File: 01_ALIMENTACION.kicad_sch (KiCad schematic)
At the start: 7 parts, among them J2 DC-005-5A-2.0, Q1 IRFR5305TRPBF, Q2 IRFR5305TRPBF

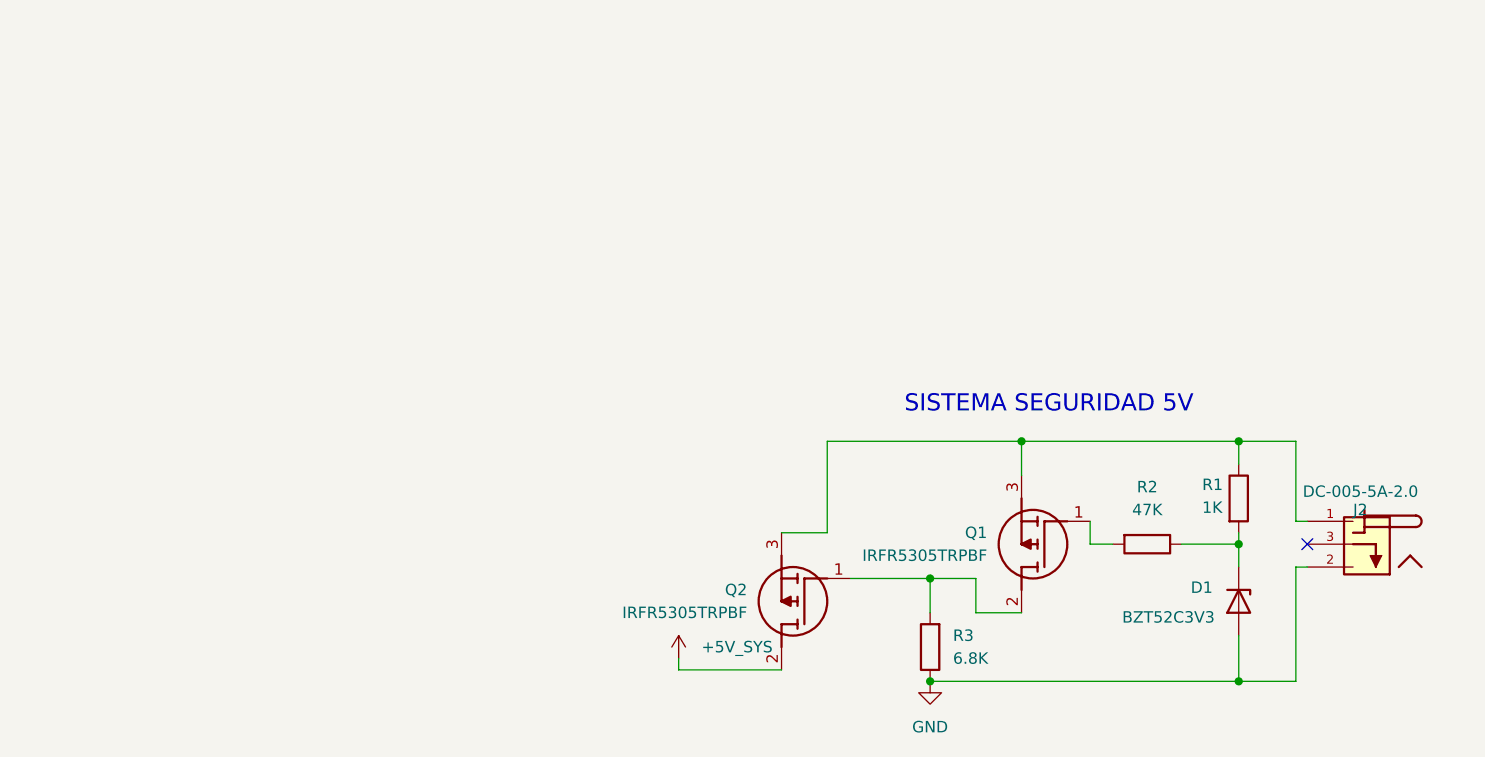
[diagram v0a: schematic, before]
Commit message: Added IMU
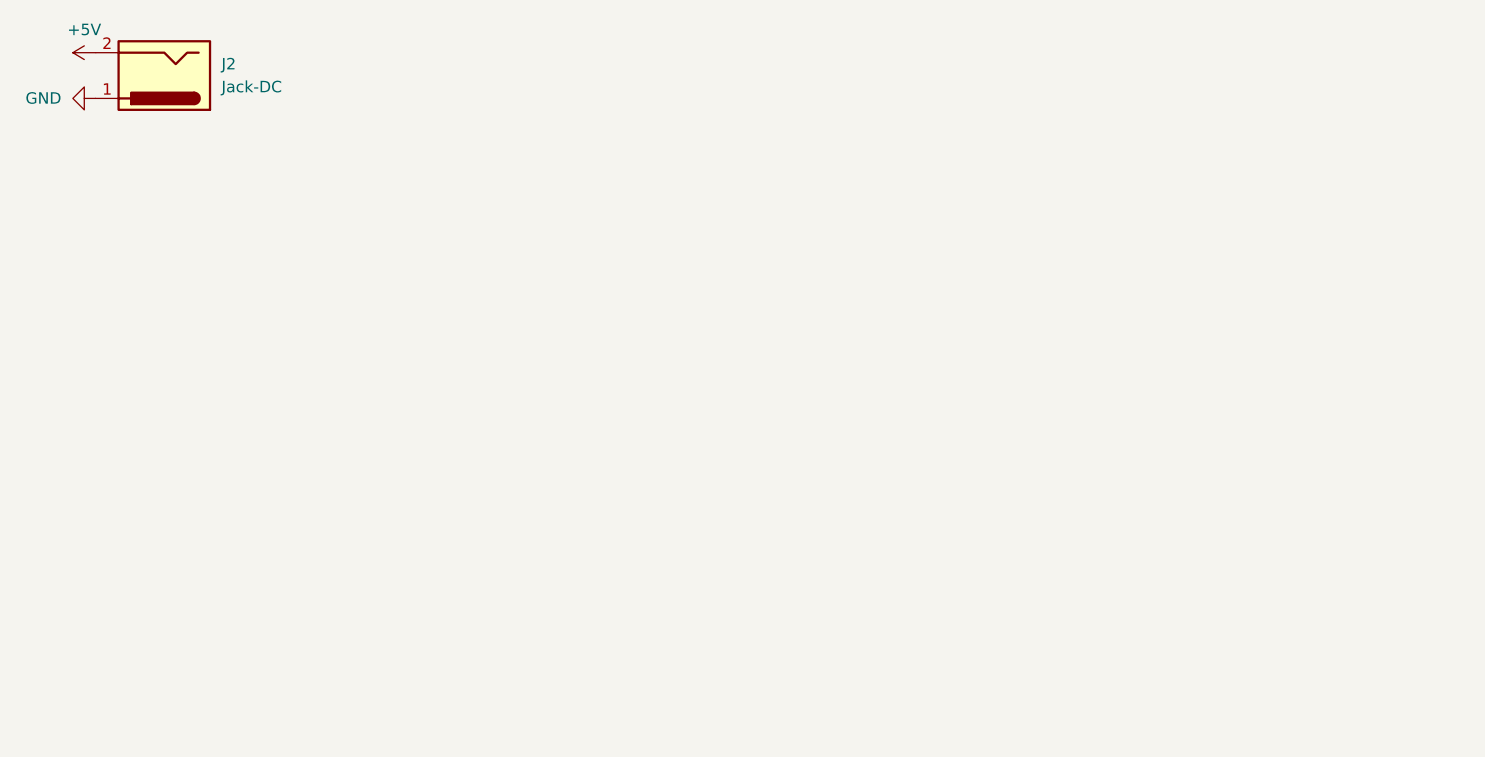
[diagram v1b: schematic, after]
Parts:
- removed D1: BZT52C3V3, Footprints:SOD3715X135N, symbol Device:D_Zener
- removed J2: DC-005-5A-2.0, Footprints:XKB_DC-005-5A-2.0, symbol Simbolos:DC-005-5A-2.0
- removed Q1, Q2: IRFR5305TRPBF, Footprints:IRFR5305TRPBF, symbol Simbolos:IRFR5305TRPBF
- removed R1: 1K, Resistor_SMD:R_0603_1608Metric, symbol Device:R
- removed R2: 47K, Resistor_SMD:R_0603_1608Metric, symbol Device:R
- removed R3: 6.8K, Resistor_SMD:R_0603_1608Metric, symbol Device:R
- added J2: Jack-DC, symbol Connector:Jack-DC
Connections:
- net GND: now also J2.1
- new net +5V: J2.2
- no-connect marks 1 -> 0
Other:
- note removed: "SISTEMA SEGURIDAD 5V"
